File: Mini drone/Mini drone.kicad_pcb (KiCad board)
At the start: 2 copper layers, 118 x 118 mm, 72 parts, among them J1 USB_C_Receptacle_USB2.0_16P, J2 JST_2mm_LiPo, J3 Conn_01x06_Socket, J4 Conn_01x06_Socket, J5 Conn_01x02_Socket, J6 Conn_01x02_Socket, J7 Conn_01x02_Socket, J8 Conn_01x02_Socket, Q1 AO3401A, SW1 SW_DPDT_x2, U1 ESP32-WROOM-32, U2 MIC5219-3.3YM5, U3 TP4056-42-ESOP8, U4 CP2102N-Axx-xQFN28, U5 DDC114TU-7-F, U6 MPU-6050, U7 DRV8833PWP, U8 DRV8833PWP, U9 PCF8574ATS

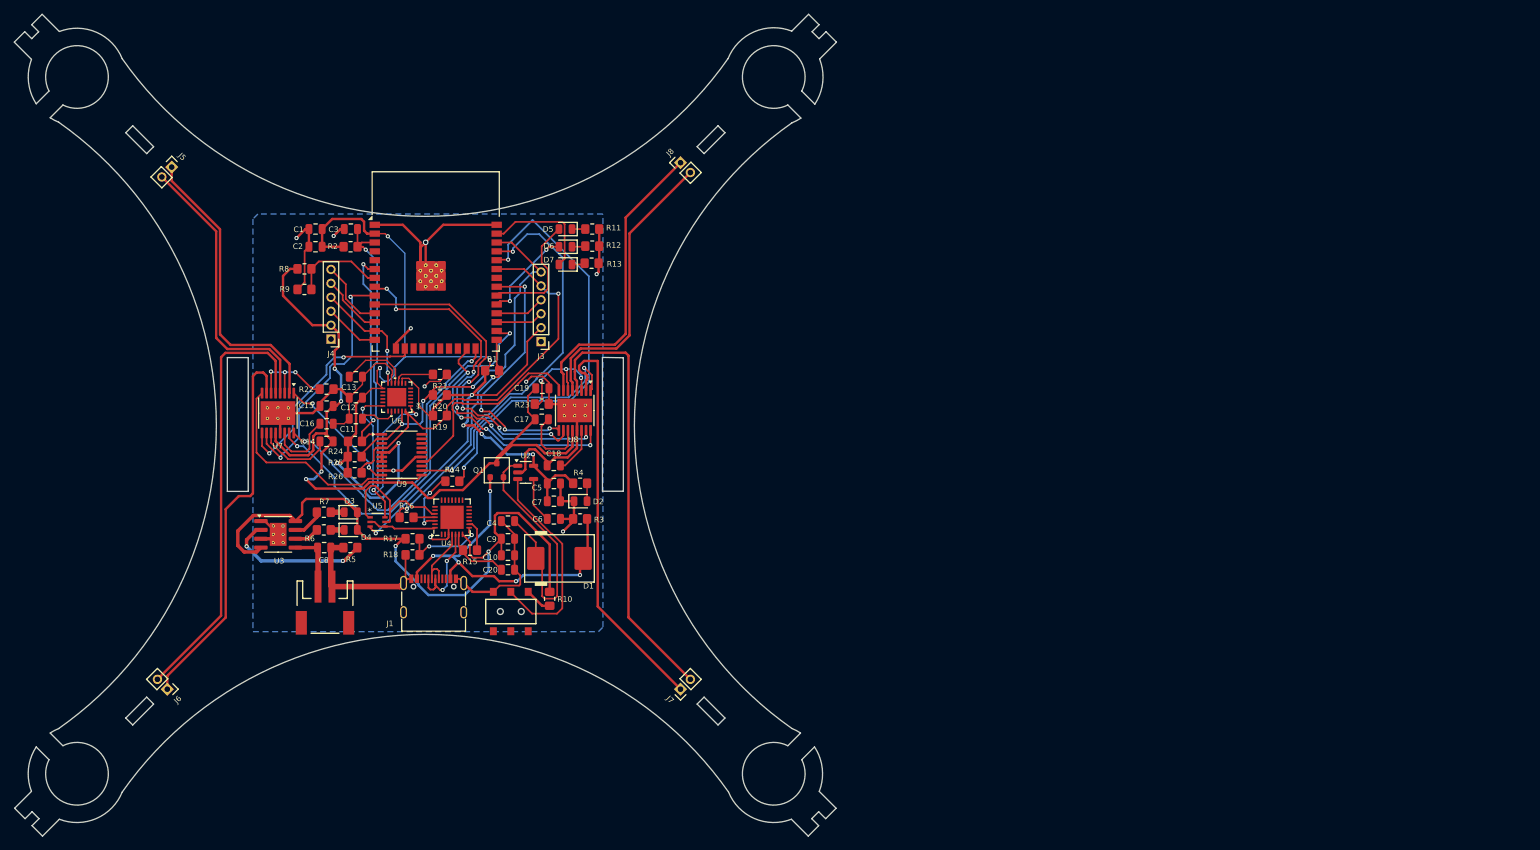
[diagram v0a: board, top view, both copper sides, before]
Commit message: 26-06-2026
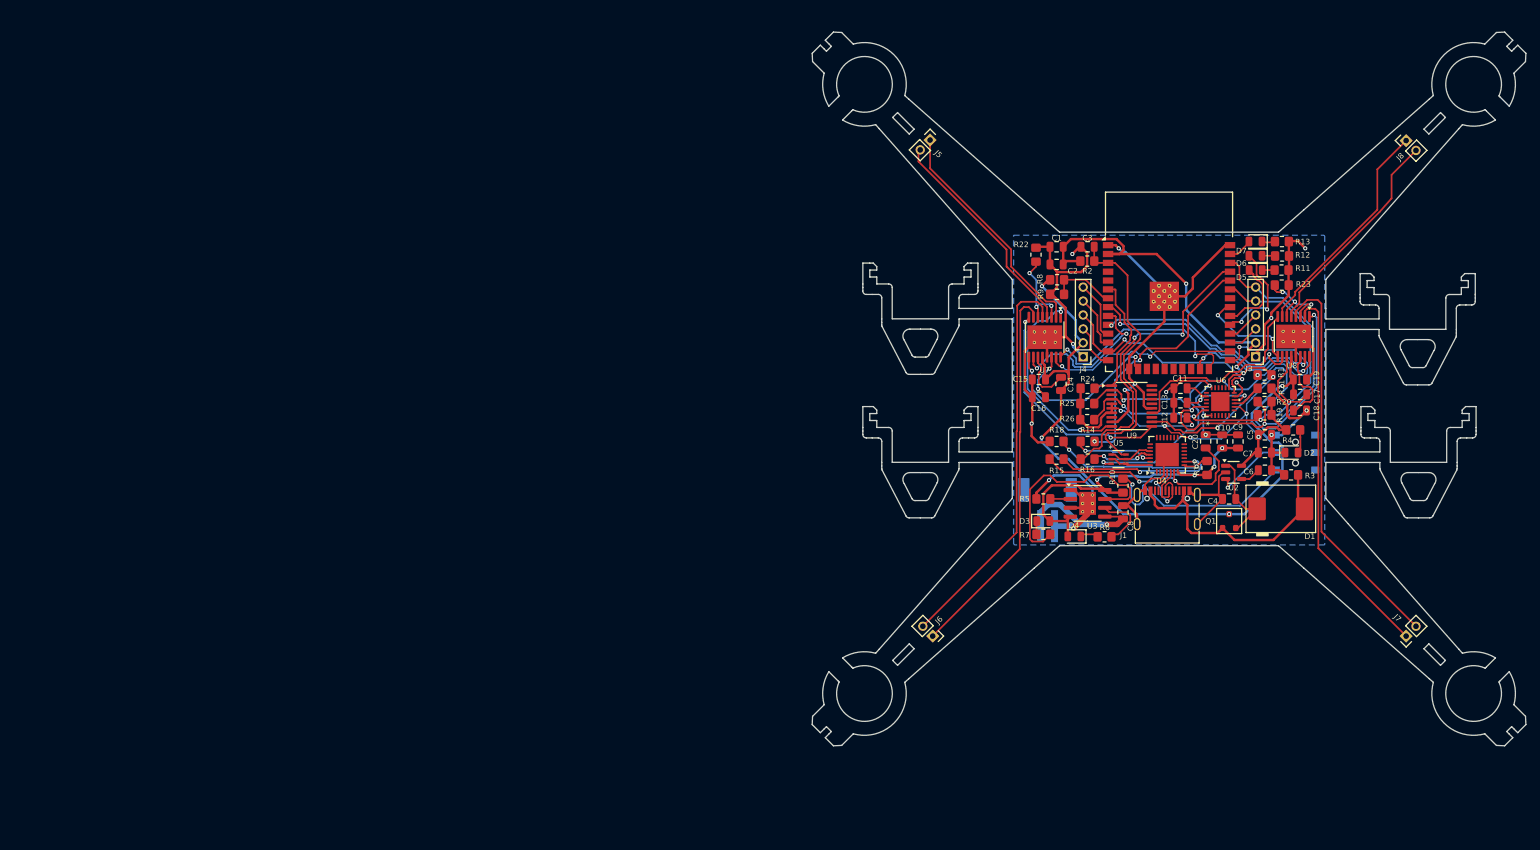
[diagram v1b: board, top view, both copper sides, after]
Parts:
- J2, SW1: moved to B.Cu
- moved C11 118.4 mm to (228.0, 102.2)
- moved C13 118.4 mm to (228.0, 104.3), turned to 0 degrees
- moved R21 118.4 mm to (240.0, 102.2)
- moved C12 118.4 mm to (227.9, 106.5)
- moved R20 118.4 mm to (240.0, 104.1)
- moved R19 118.4 mm to (240.0, 106.0), turned to 0 degrees
- moved U6 118.2 mm to (233.7, 104.1), turned to 90 degrees
- moved U3 116.3 mm to (214.6, 118.7)
- moved SW1 114.9 mm to (244.5, 111.4), turned to 0 degrees
- moved C8 114.8 mm to (219.7, 120.0), turned to 90 degrees
- moved R17 114.5 mm to (231.8, 113.7), turned to 90 degrees
- moved R6 112.1 mm to (217.1, 123.5), turned to 0 degrees
- moved R1 110.9 mm to (240.0, 100.3), turned to 180 degrees
- moved U7 110.6 mm to (208.5, 94.9)
- moved J6 110.1 mm to (192.4, 137.8)
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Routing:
- net VBUS: track 93.2 -> 50.7 mm, vias 2 -> 4
- net 3.3V: track 169.9 -> 130.5 mm, vias 9 -> 10
- net /B_MOT_1: track 57.4 -> 27.9 mm
- net Net-(U3-~{CHRG}): track 4.54 -> 32.4 mm
- net Net-(SW1A-C): track 3.91 -> 30.9 mm, vias 0 -> 1
- net /RX: track 62.6 -> 36.2 mm
- net Net-(D1-K): track 38.3 -> 13.6 mm
- net Net-(U4-VDD): track 9.48 -> 32.9 mm, vias 0 -> 2
- net /A_MOT_4: track 37.2 -> 14.3 mm, vias 4 -> 2
- net /IO0: track 37.0 -> 58.0 mm, vias 2 -> 3
- net /motor_driver/Sl2: track 36.1 -> 56.1 mm
- net LDD_EN: track 30.3 -> 10.3 mm, vias 0 -> 1
- net Net-(U4-~{RST}): track 4.45 -> 23.9 mm, vias 0 -> 2
- net /SCL: track 54.7 -> 73.4 mm
- net Net-(U3-PROG): track 21.1 -> 2.88 mm, vias 2 -> 0
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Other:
- board size 118 x 118 mm -> 102.4 x 102.4 mm
